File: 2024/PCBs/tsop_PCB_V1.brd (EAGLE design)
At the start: 60 x 60 mm, 84 parts, among them IC2 CD74HC4067SM96, Q1 BSS138

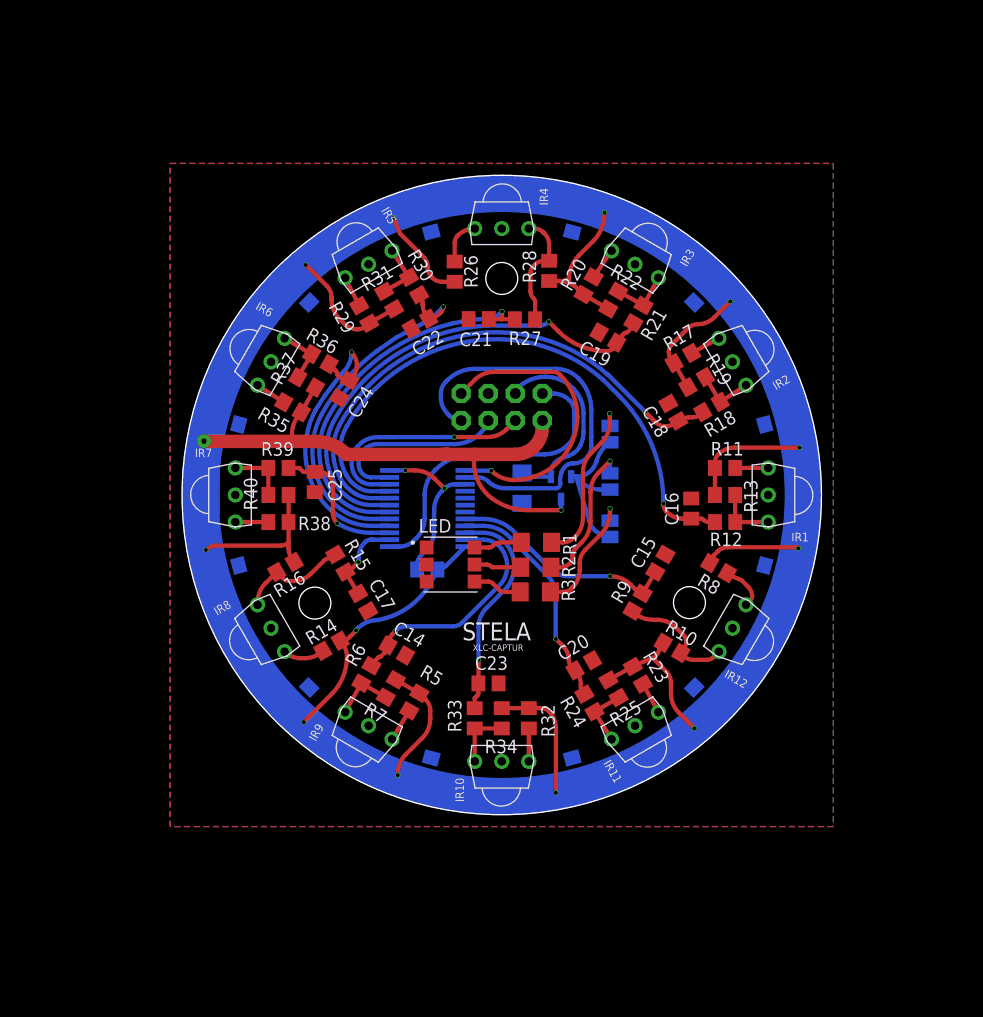
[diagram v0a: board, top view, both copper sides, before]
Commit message: tsopV1
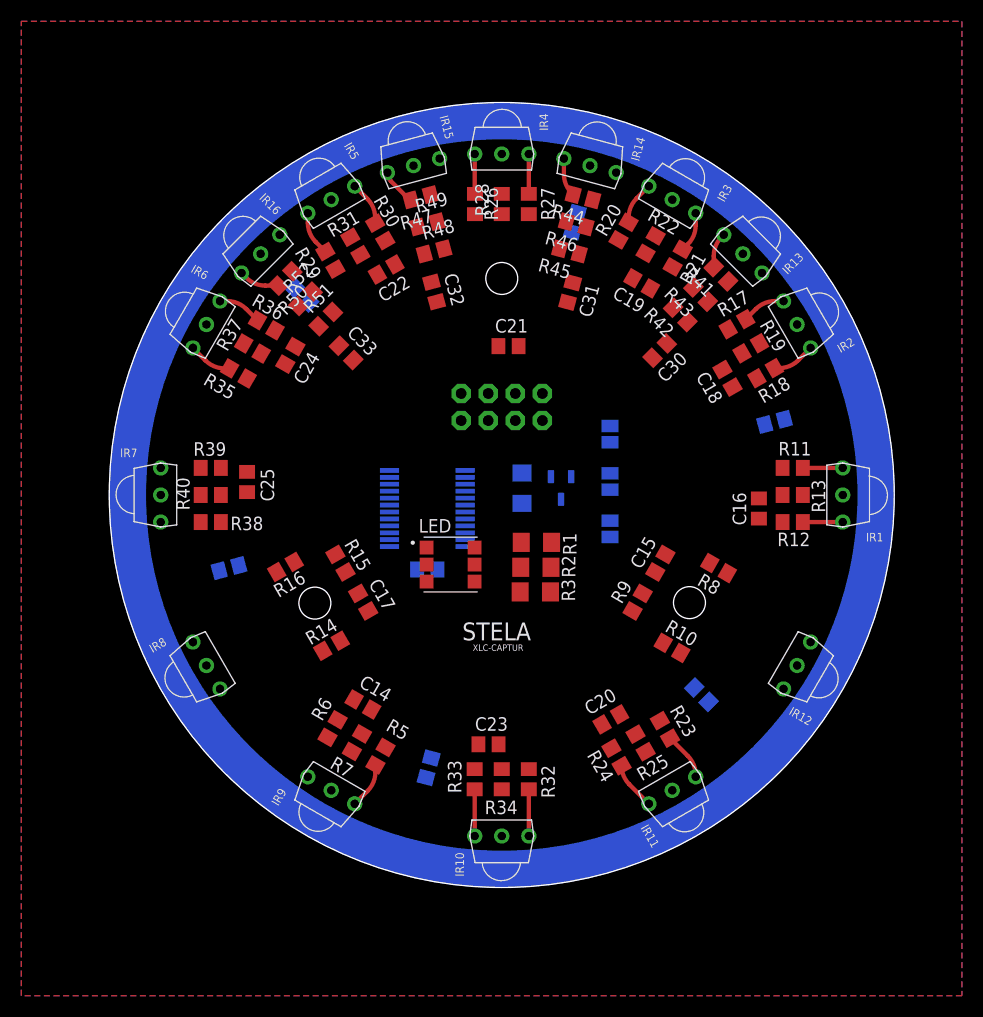
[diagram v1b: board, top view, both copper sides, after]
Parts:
- removed C11, C13, C3, C5, C7, C9: 100nF, rcl:C0805
- added C30, C31, C32, C33: 1u, rcl:C0805
- added IR13, IR14, IR15, IR16: TSSP58038, TSOP4038:TSOP
- added R41, R44, R47, R50: 10R, rcl:R0805
- added R42, R45, R48, R51: 100k, rcl:R0805
- added R43, R46, R49, R52: 4.7k, rcl:R0805
- C14, C15, C16: value (none) -> 1u
- R10, R13, R7: value (none) -> 4.7k
- R11, R5, R8: value (none) -> 10R
- R12, R6, R9: value (none) -> 100k
- moved R27 10.8 mm to (2.54, 27.3), turned to 90 degrees
- moved R28 7.69 mm to (0.00, 27.3)
- moved IR11 7.00 mm to (16.0, -27.7)
- moved IR12 7.00 mm to (27.7, -16.0)
- moved IR2 7.00 mm to (27.7, 16.0)
- moved IR3 7.00 mm to (16.0, 27.7)
- moved IR5 7.00 mm to (-16.0, 27.7)
- moved IR6 7.00 mm to (-27.7, 16.0)
- moved IR8 7.00 mm to (-27.7, -16.0)
- moved IR9 7.00 mm to (-16.0, -27.7)
- moved IR1 7.00 mm to (32.0, 0.00)
- moved IR10 7.00 mm to (0.00, -32.0)
- moved IR4 7.00 mm to (0.00, 32.0)
- moved IR7 7.00 mm to (-32.0, 0.00)
- moved R26 6.63 mm to (-2.51, 27.3)
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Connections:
- new net N$24: IR13.VS, R41.2
- new net N$28: IR14.VS, R44.2
- new net N$31: IR15.VS, R47.2
- new net N$33: IR16.VS, R50.2
- new net N$35: IR13.VO, R42.2, R43.2
- new net N$37: IR14.VO, R45.2, R46.2
- new net N$38: IR15.VO, R48.2, R49.2
- new net N$39: IR16.VO, R51.2, R52.2
- net +5V: now also R41.1, R43.1, R44.1, R46.1, R47.1, R49.1, R50.1, R52.1; no longer C11.1, C13.1, C3.1, C5.1, C7.1, C9.1
- net GND: now also C30.2, C31.2, C32.2, C33.2, IR13.GND, IR14.GND, IR15.GND, IR16.GND; no longer C11.2, C13.2, C3.2, C5.2, C7.2, C9.2
- net I12: now also C30.1, R42.1
- net I13: now also C31.1, R45.1
- net I14: now also C32.1, R48.1
- net I15: now also C33.1, R51.1
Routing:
- net +5V: track 378.0 -> 0.00 mm, vias 14 -> 0
- net I0: track 55.5 -> 0.00 mm, vias 1 -> 0
- net I1: track 50.7 -> 0.00 mm, vias 1 -> 0
- net I2: track 45.0 -> 0.00 mm, vias 1 -> 0
- net LIGHT_SET_2: track 38.5 -> 0.00 mm
- net I3: track 35.9 -> 0.00 mm, vias 1 -> 0
- net I4: track 34.0 -> 0.00 mm, vias 1 -> 0
- net IR_READ: track 29.5 -> 0.00 mm
- net I5: track 27.6 -> 0.00 mm, vias 1 -> 0
- net LIGHT_SET_3: track 27.4 -> 0.00 mm, vias 1 -> 0
- net I8: track 22.6 -> 0.00 mm, vias 1 -> 0
- net LIGHT_SET_0: track 21.6 -> 0.00 mm, vias 1 -> 0
- net I10: track 21.5 -> 0.00 mm, vias 1 -> 0
- net I11: track 21.2 -> 0.00 mm, vias 1 -> 0
- net I9: track 20.6 -> 0.00 mm, vias 1 -> 0
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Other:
- board size 60 x 60 mm -> 73.7 x 73.7 mm
